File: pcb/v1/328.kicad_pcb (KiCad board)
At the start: 2 copper layers, 69.8 x 43.2 mm, 31 parts, among them J1 USB C, J2 CONNECTS TO GPS, J3 Battery Connection, J5 Conn_01x05, J6 SD Card, SW1 SW_Push, U1 MSP MCU, U2 USB TO UART, U3 Low Dropout Regulator, U4 RFM95W-915S2, U5 BME680, Y1 Crystal

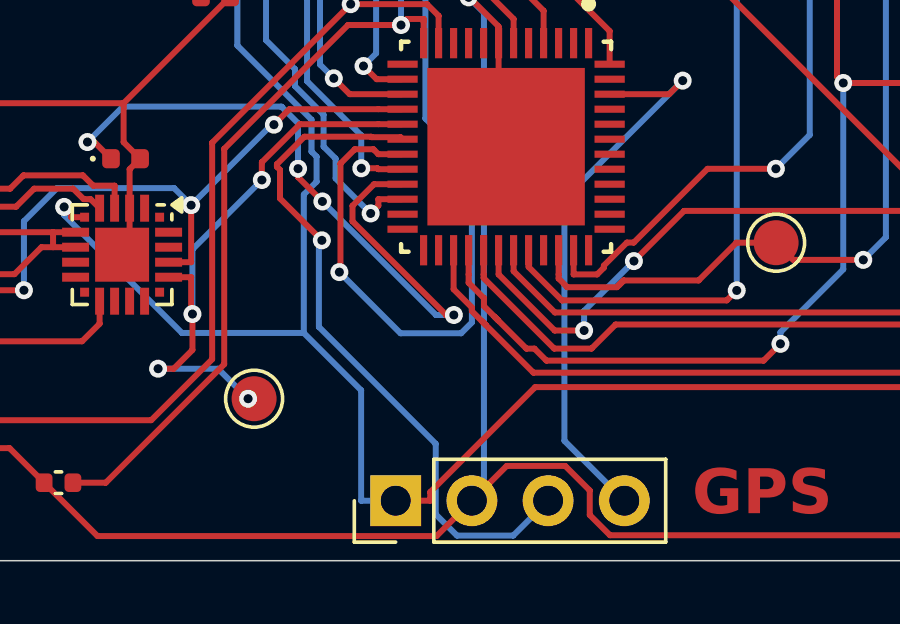
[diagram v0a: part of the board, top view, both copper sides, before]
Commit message: pcb updates
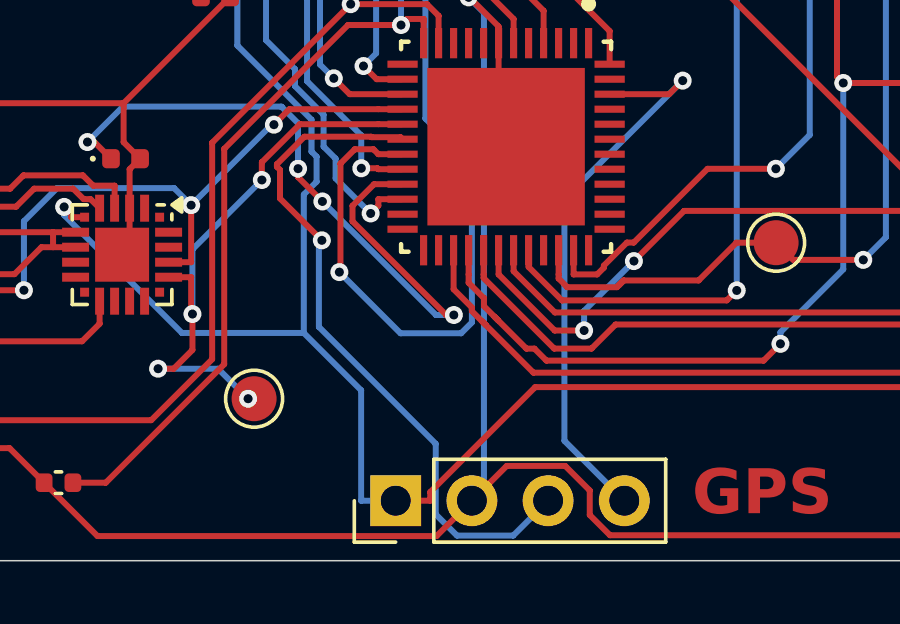
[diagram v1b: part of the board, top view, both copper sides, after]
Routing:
- net /LED_GPS: track 26.5 -> 25.8 mm
